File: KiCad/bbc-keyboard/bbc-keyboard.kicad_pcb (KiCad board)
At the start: 2 copper layers, 337.8 x 137.2 mm, 104 parts, among them IC1 74LS161, IC2 74251, IC3 74145, IC4 74LS30, SW1 escape, SW10 W, SW11 2, SW12 A, SW13 S, SW14 Z, SW15 f2, SW16 4, SW17 E, SW18 D, SW19 X, SW2 Q, SW20 C, SW21 space, SW22 f3, SW23 5, SW24 T, SW25 R, SW26 F, SW27 G, SW28 V, SW29 f5, SW3 F0, SW30 F4, SW31 7, SW32 6, SW33 Y, SW34 H, SW35 B, SW36 f6, SW37 8, SW38 9, SW39 U, SW4 1, SW40 J, SW41 N, SW42 M, SW43 f8, SW44 f7, SW45 I, SW46 O, SW47 K, SW48 L, SW49 <,, SW5 caps lk, SW50 f9, SW51 =-, SW52 0, SW53 P, SW54 @, SW55 ;+, SW56 >., SW57 \|, SW58 ~^, SW59 _£, SW6 shift lk, SW60 {[, SW61 *:, SW62 }], SW63 ?/, SW64 right, SW65 left, SW66 down, SW67 up, SW68 return, SW69 delete, SW7 tab, SW70 copy, SW71 shift, SW72 shift, SW73 ctrl, SW74 SW_DIP_x08, SW75 break, SW8 f1, SW9 3

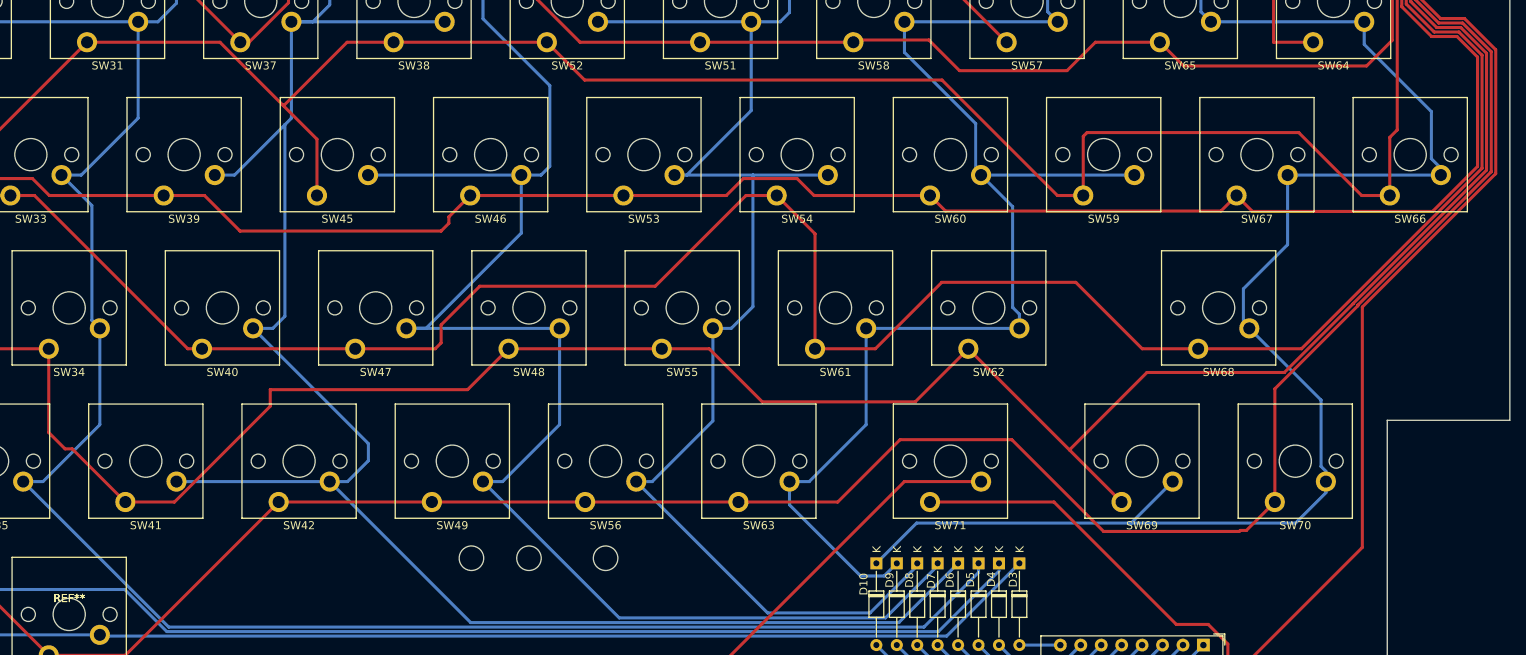
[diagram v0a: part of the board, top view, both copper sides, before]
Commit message: return stabilizers
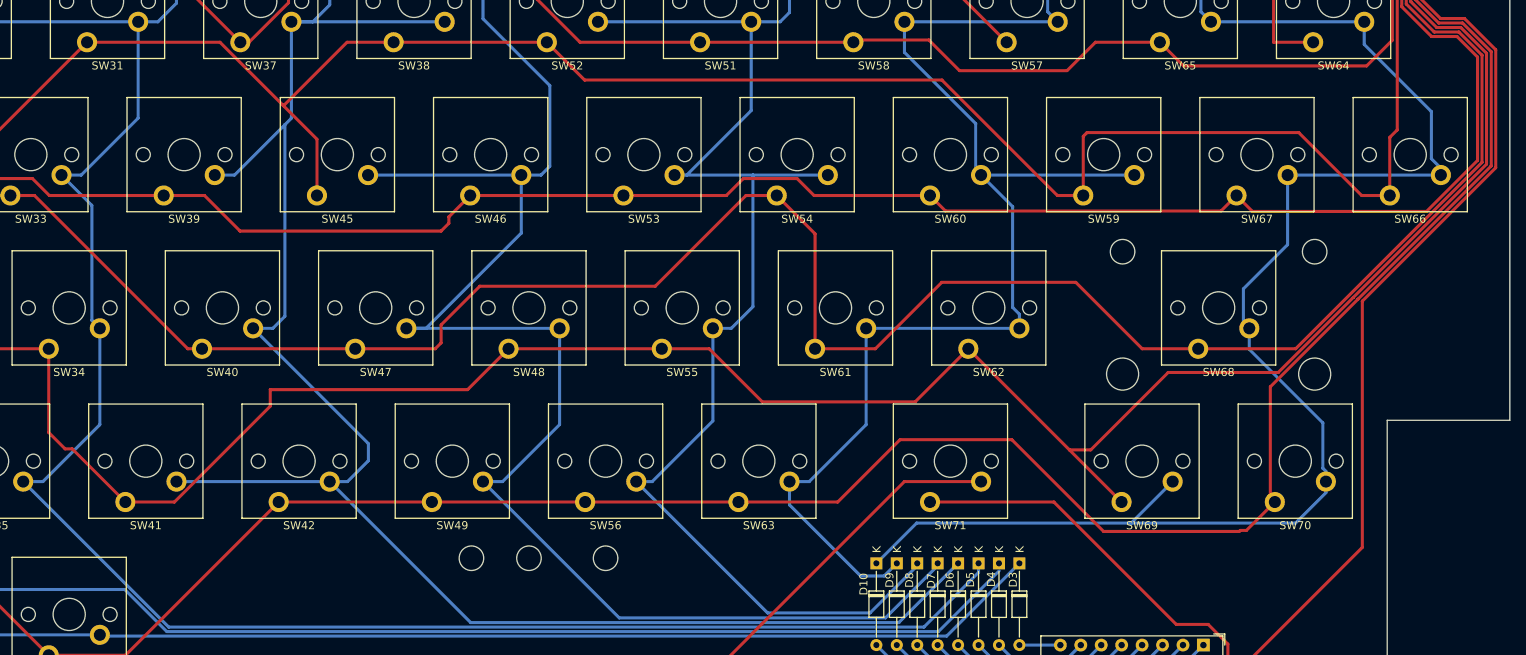
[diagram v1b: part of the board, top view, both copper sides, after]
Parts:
- added REF**: Stabilizer_Cherry_MX_2.00u, Mounting_Keyboard_Stabilizer:Stabilizer_Cherry_MX_2.00u, F.Cu at (347.7, 177.8)
